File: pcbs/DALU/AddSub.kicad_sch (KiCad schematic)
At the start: 8 parts, among them U401 74HC86, U402 74HC86, U403 74HC86, U404 74HC08, U405 74HC283, U406 74HC283, U407 74HC245, U408 74HC245

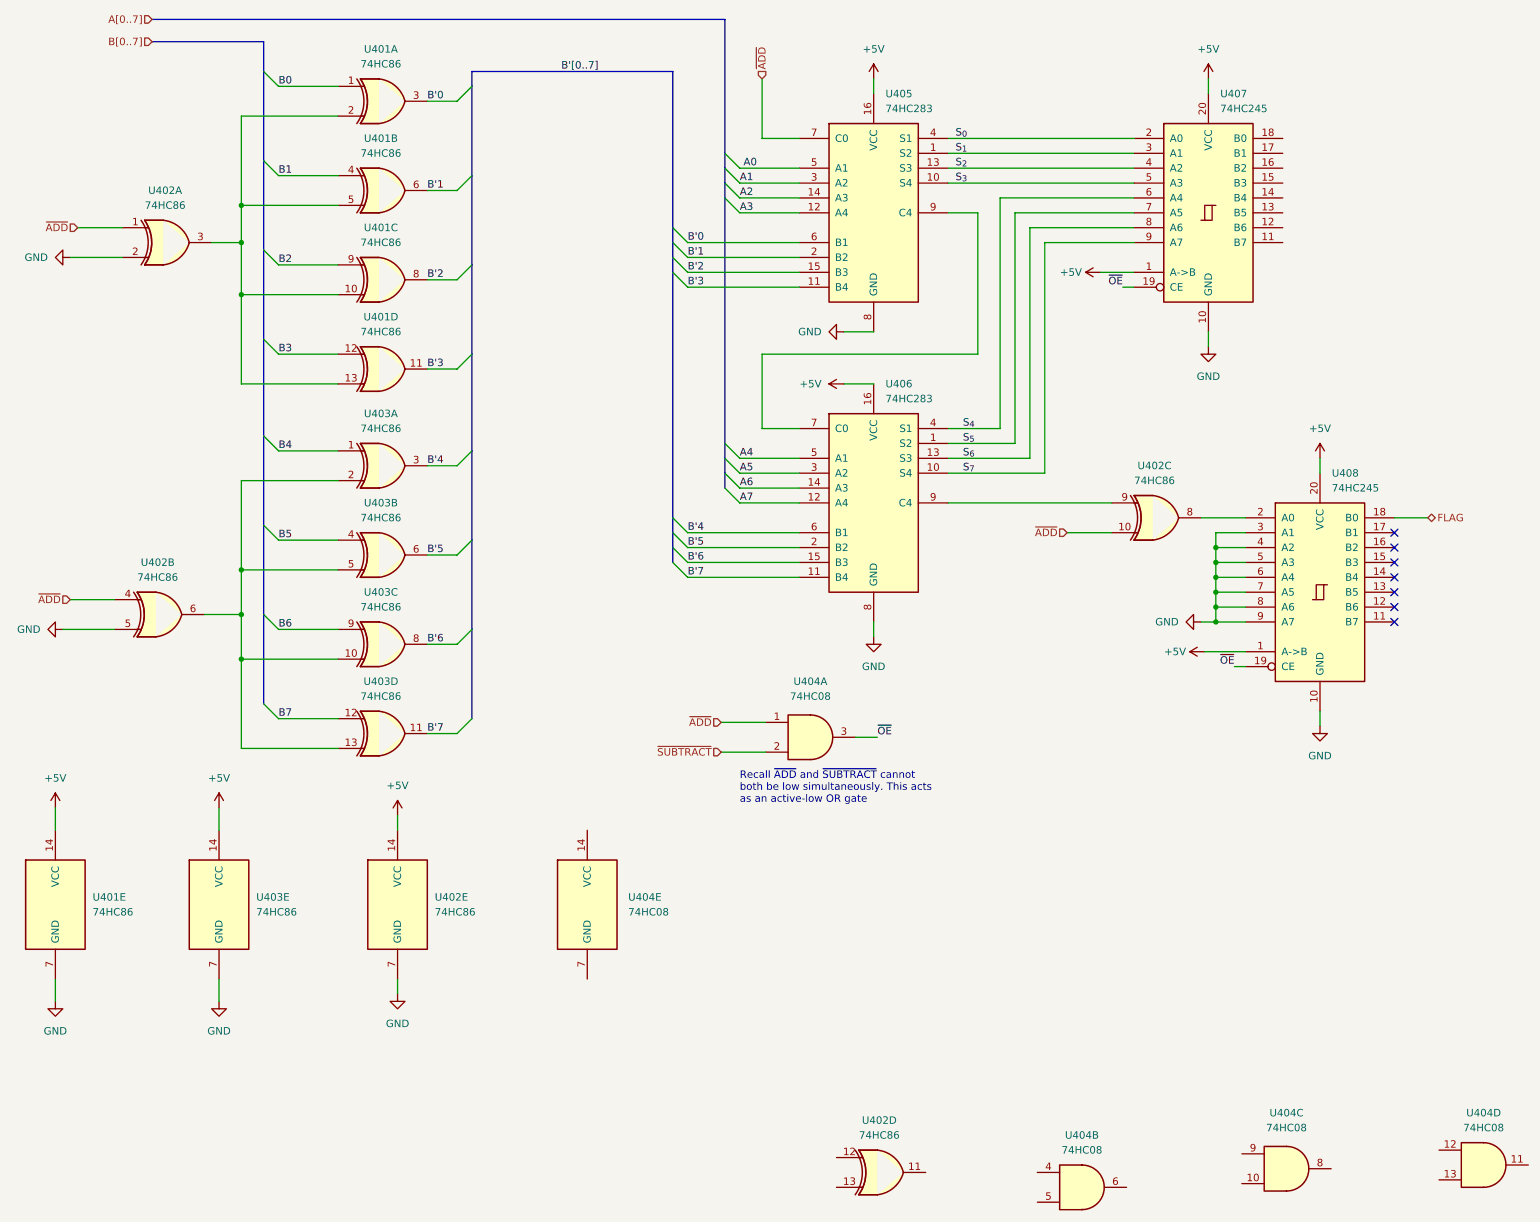
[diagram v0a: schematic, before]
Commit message: Fixing a lot of routing
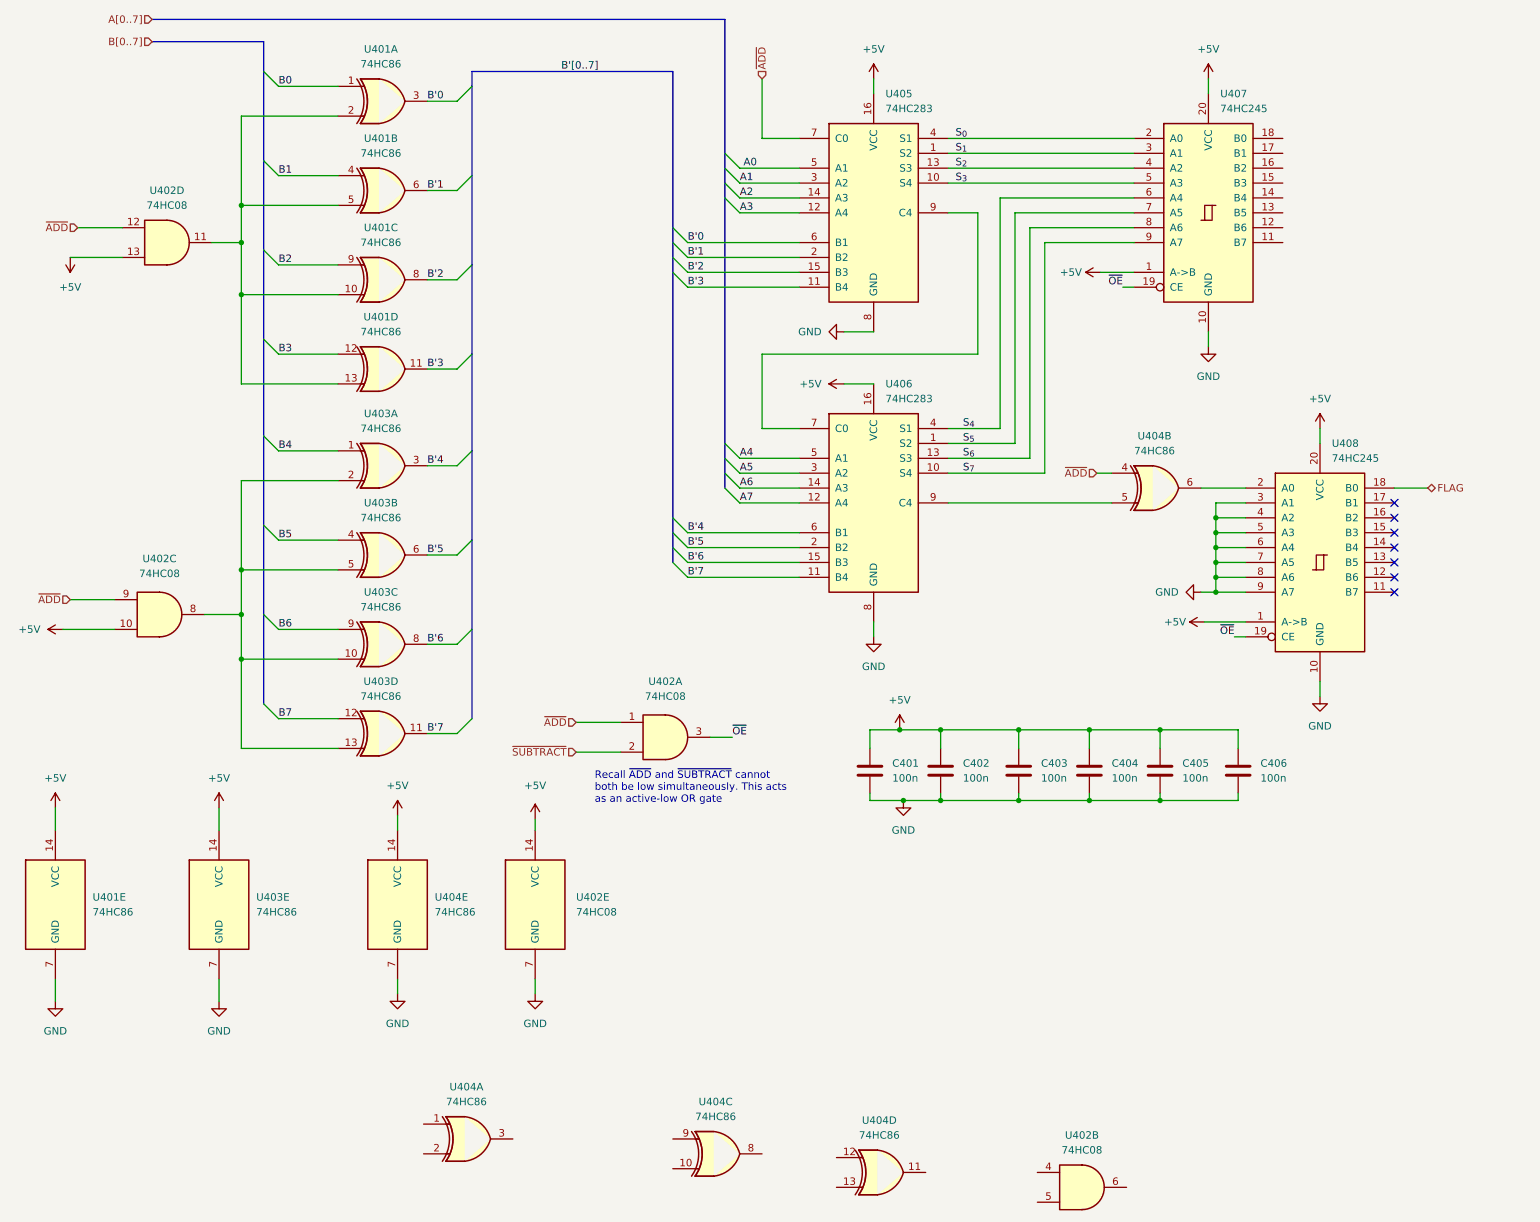
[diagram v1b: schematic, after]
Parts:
- added C401, C402, C403, C404, C405, C406: 100n, Capacitor_SMD:C_0603_1608Metric, symbol Device:C
- renumbered U404 to U402, U402 to U404
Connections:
- net +5V: now also U402.10, U402.13, U402.14 (VCC), C401.1, C402.1, C403.1, C404.1, C405.1, C406.1
- net GND: now also U402.7 (GND), C401.2, C402.2, C403.2, C404.2, C405.2, C406.2; no longer U404.2, U404.5
- net ~{ADD}: now also U402.12, U402.9; no longer U404.1, U404.10
- net at U408.2 (A0): now also U404.6; no longer U404.8
- net at U404.9: no longer U406.9 (C4)
- net at U401.10, U401.13, U401.2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: now also U402.11; no longer U404.3
- net at U403.10, U403.13, U403.2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: now also U402.8; no longer U404.6
- new net: U404.5, U406.9 (C4)
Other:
- moved on the sheet: U402A, U402C, U402D, U402E, U404A, U404B, U404C, U408
